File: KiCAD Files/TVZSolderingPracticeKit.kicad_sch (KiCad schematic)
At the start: 49 parts, among them J1 Barrel Jack, J2 Conn_01x05_Pin, J3 Conn_01x05_Socket, J4 Conn_01x03_Pin, J5 Conn_01x03_Pin, J6 JUMPER-H/R, J7 JUMPER-H/B, SW1 SW_Push, SW10 POWER, SW11 C/D, SW2 SW_Push, SW3 SW_Push, SW4 SW_Push, SW5 SW_Push, SW6 SW_Push, SW7 SW_Push, SW8 SW_Push, U1 NE555P

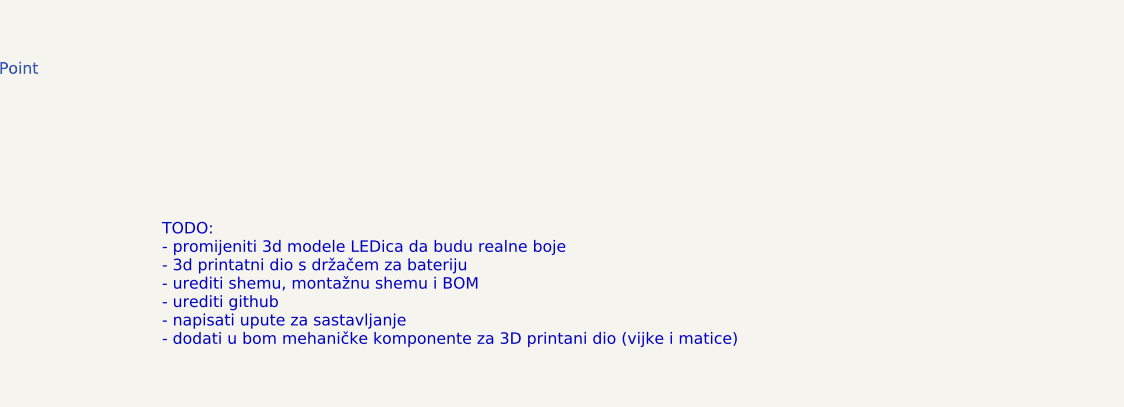
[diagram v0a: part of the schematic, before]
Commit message: update
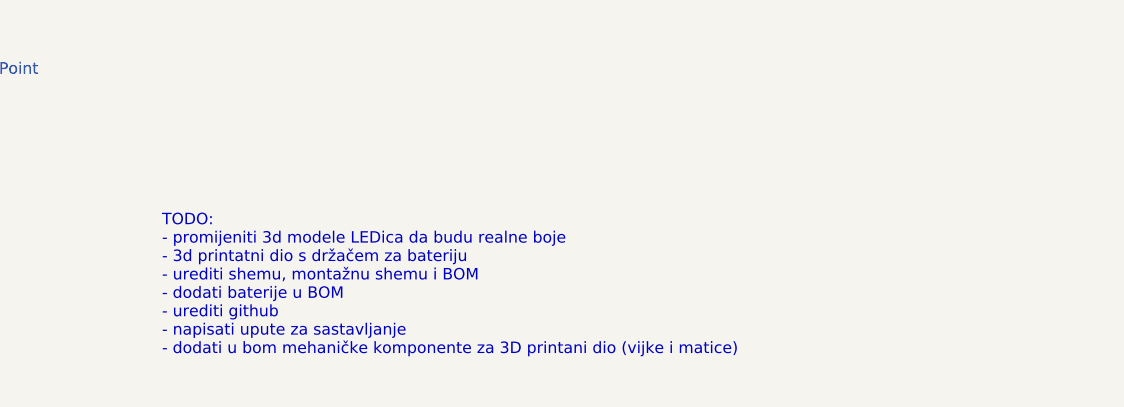
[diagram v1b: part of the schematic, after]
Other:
- note added: "TODO: - promijeniti 3d modele LEDica da budu realne boje - 3d printatni dio s držačem za bateriju - urediti shemu, montažnu shemu i BOM - dodati baterije u BOM - urediti github - napisati upute za sastavljanje - dodati u bom mehaničke komponente za 3D printani dio (vijke i matice)"
- note removed: "TODO: - promijeniti 3d modele LEDica da budu realne boje - 3d printatni dio s držačem za bateriju - urediti shemu, montažnu shemu i BOM - urediti github - napisati upute za sastavljanje - dodati u bom mehaničke komponente za 3D printani dio (vijke i matice)"
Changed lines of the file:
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@@
 	(generator_version "9.0")
 	(paper "A4")
-	(text "TODO:\n- promijeniti 3d modele LEDica da budu realne boje\n- 3d printatni dio s držačem za bateriju\n- urediti shemu, montažnu shemu i BOM\n- urediti github\n- napisati upute za sastavljanje\n- dodati u bom mehaničke komponente za 3D printani dio (vijke i matice)"
+	(text "TODO:\n- promijeniti 3d modele LEDica da budu realne boje\n- 3d printatni dio s držačem za bateriju\n- urediti shemu, montažnu shemu i BOM\n- dodati baterije u BOM\n- urediti github\n- napisati upute za sastavljanje\n- dodati u bom mehaničke komponente za 3D printani dio (vijke i matice)"
 		(exclude_from_sim no)
 		(at 86.614 174.498 0)
